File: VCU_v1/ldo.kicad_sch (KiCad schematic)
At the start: 6 parts, among them U2 AMS1117-3.3, U7 MIC5200-4.8YS

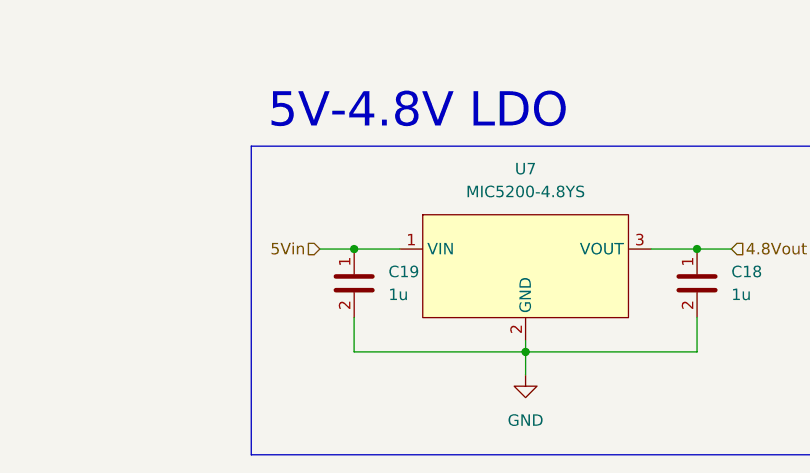
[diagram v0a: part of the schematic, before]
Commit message: p dih r
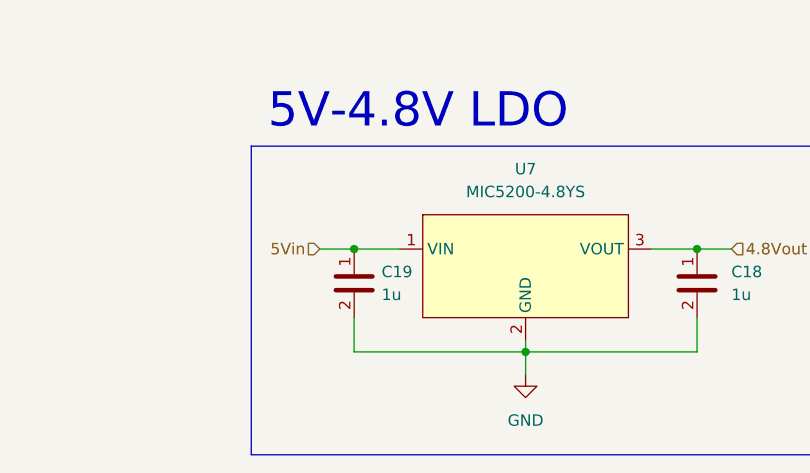
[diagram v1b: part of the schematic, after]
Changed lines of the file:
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@@
 		(on_board yes)
 		(dnp no)
-		(fields_autoplaced yes)
 		(property "Reference" "C19"
-			(at 110.49 113.0299 0)
+			(at 109.728 113.03 0)
 			(effects
 				(font
@@
 		)
 		(property "Value" "1u"
-			(at 110.49 115.5699 0)
+			(at 109.728 115.57 0)
 			(effects
 				(font
